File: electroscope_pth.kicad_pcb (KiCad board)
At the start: 2 copper layers, 25.3 x 46.6 mm, 17 parts, among them Q1 Q_PNP_EBC, Q2 Q_NPN_EBC, Q3 Q_PNP_EBC, Q4 Q_NPN_EBC, Q5 Q_PNP_EBC, Q6 Q_NPN_EBC, U1 ANT, U2 ANT

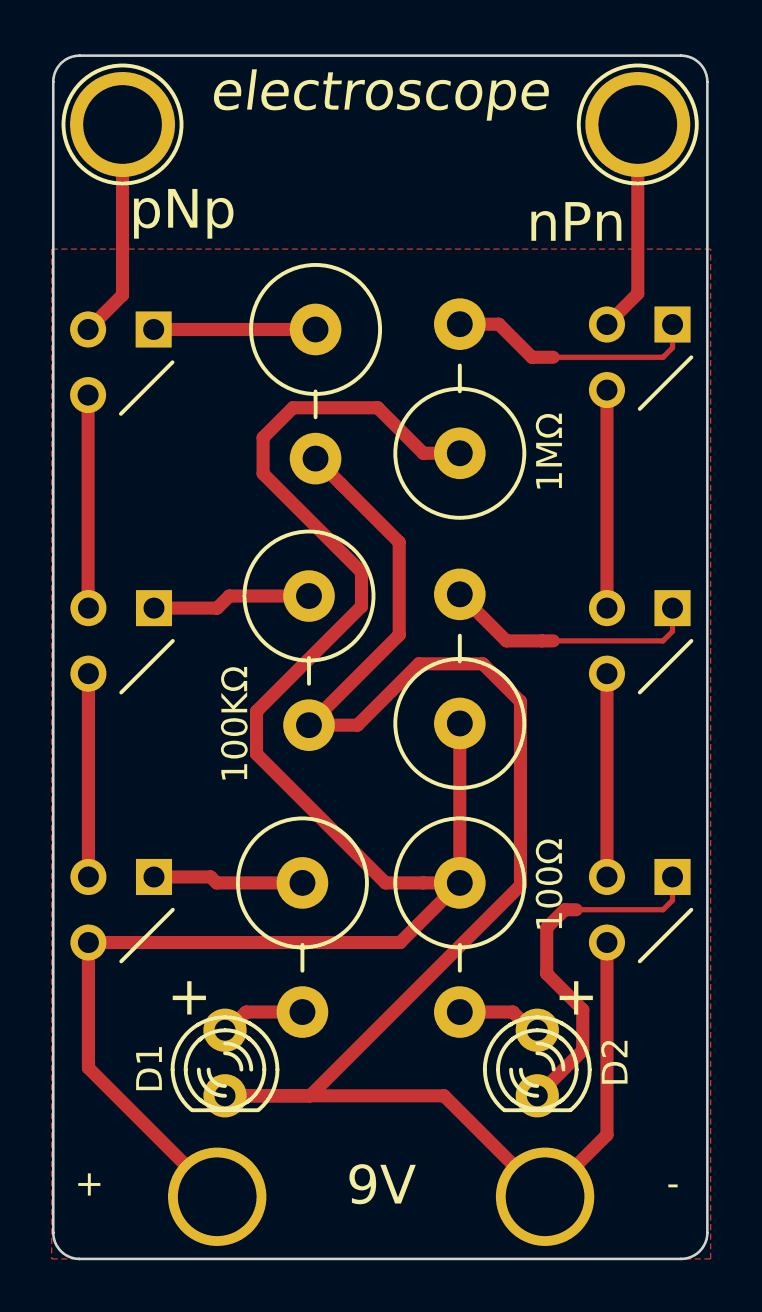
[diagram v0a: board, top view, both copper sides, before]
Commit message: More rounding and compaction
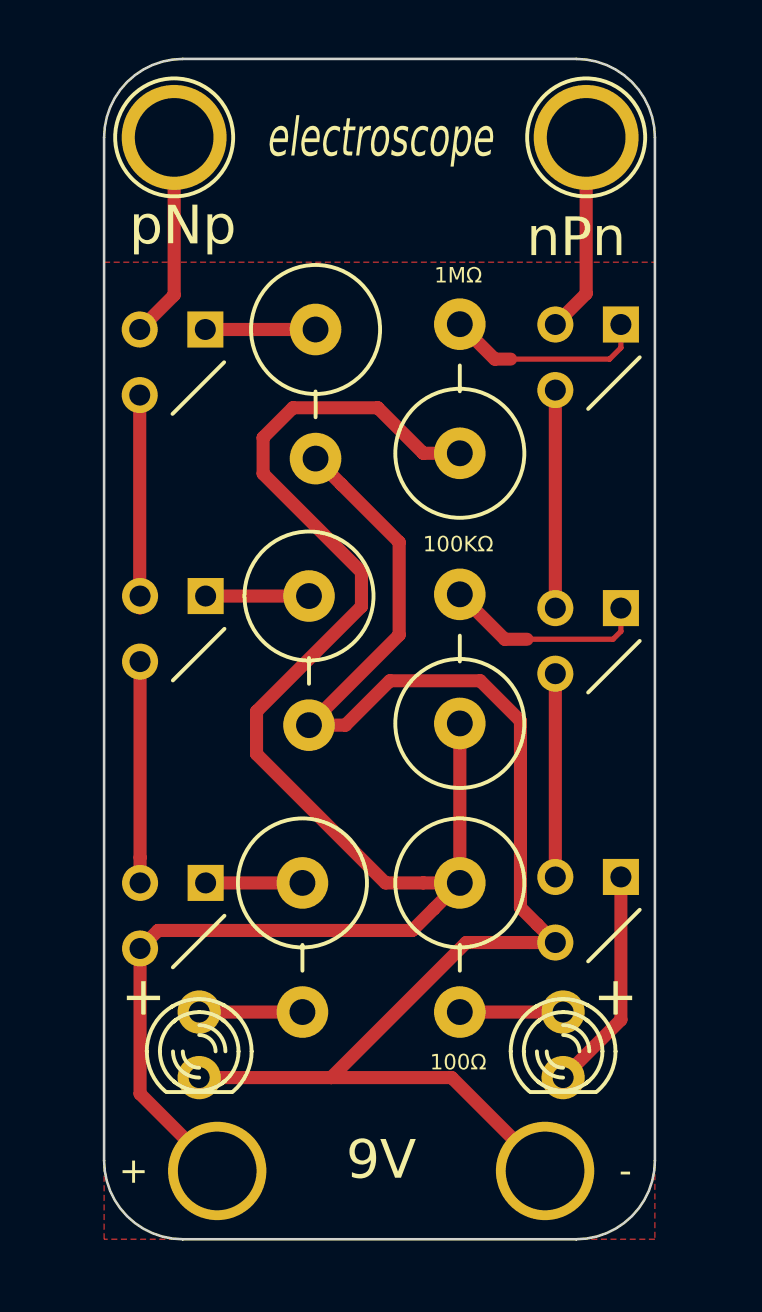
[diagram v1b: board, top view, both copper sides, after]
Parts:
- moved U1 2.06 mm to (147.7, 71.4)
- moved U2 2.06 mm to (131.7, 71.4)
- moved Q3 2.05 mm to (131.7, 90.4)
- moved Q1 2.01 mm to (131.7, 101.5)
- moved Q2 2.00 mm to (147.8, 79.9)
- moved Q4 2.00 mm to (147.8, 90.9)
- moved Q5 2.00 mm to (131.7, 80.1)
- moved Q6 2.00 mm to (147.8, 101.3)
- moved D1 1.22 mm to (132.7, 106.5)
- moved D2 1.22 mm to (146.8, 106.5)
- moved BT1 1.00 mm to (139.8, 111.5)
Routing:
- net GND: track 69.7 -> 57.6 mm
- net Net-(D2-Pad2): track 14.0 -> 8.70 mm
- net VCC: track 67.7 -> 63.8 mm
- net Net-(Q3-Pad3): track 6.20 -> 4.00 mm
- net Net-(Q1-Pad3): track 5.85 -> 3.75 mm
- net Net-(Q4-Pad3): track 10.0 -> 7.99 mm
- net Net-(Q5-Pad3): track 6.27 -> 4.27 mm
- net Net-(Q2-Pad3): track 9.83 -> 7.88 mm
- net Net-(D2-Pad1): track 3.29 -> 4.00 mm
- net Net-(D1-Pad1): track 3.29 -> 4.00 mm
- net Net-(Q1-Pad2): track 7.87 -> 8.57 mm
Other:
- board size 25.3 x 46.6 mm -> 21.3 x 45.7 mm
